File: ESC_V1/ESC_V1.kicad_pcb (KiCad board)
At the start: 2 copper layers, 58.2 x 22.2 mm, 19 parts, among them J1 Conn_01x07_Female, J2 Conn_01x01_Female, J3 Conn_01x01_Female, J4 Conn_01x01_Female, J5 Conn_01x01_Female, J6 Conn_01x01_Female, Q1 BSP129, Q11 P Channel 40V 30A, Q2 BSP129, Q3 P Channel 40V 30A, Q4 BSP129, Q7 P Channel 40V 30A, U1 ULN2803A

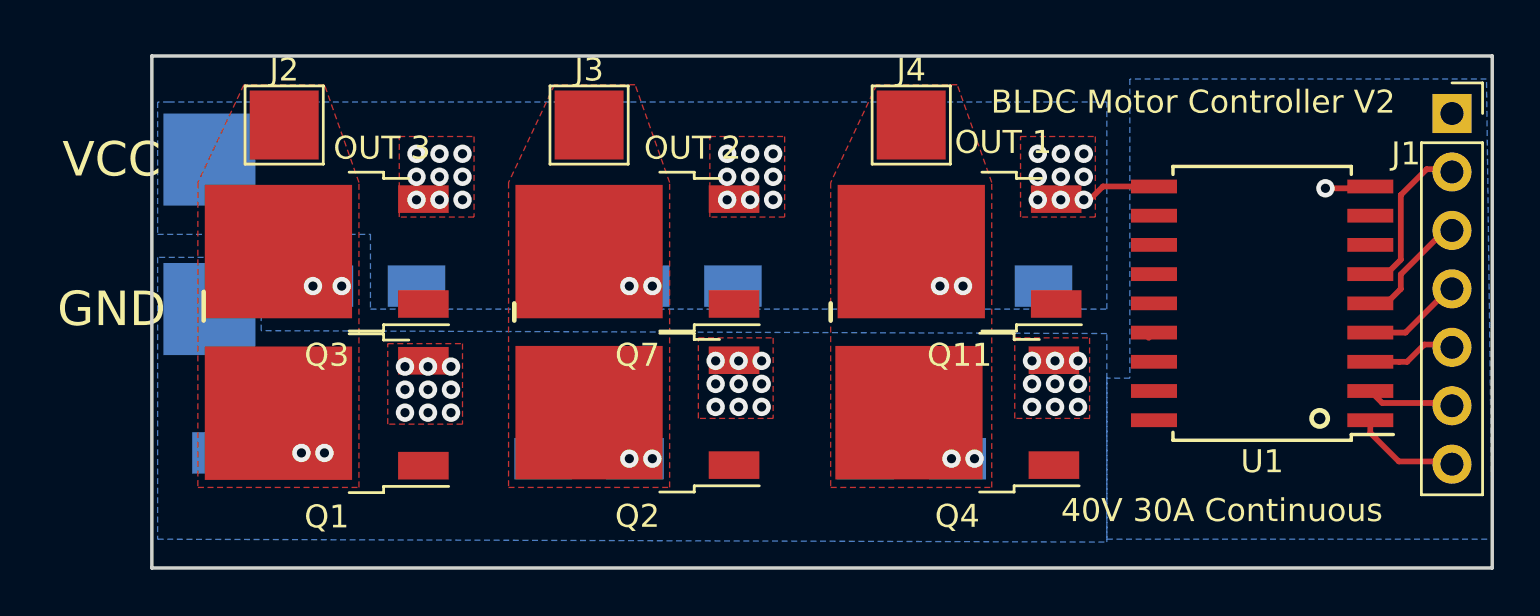
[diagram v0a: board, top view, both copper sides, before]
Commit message: Fixing git issues
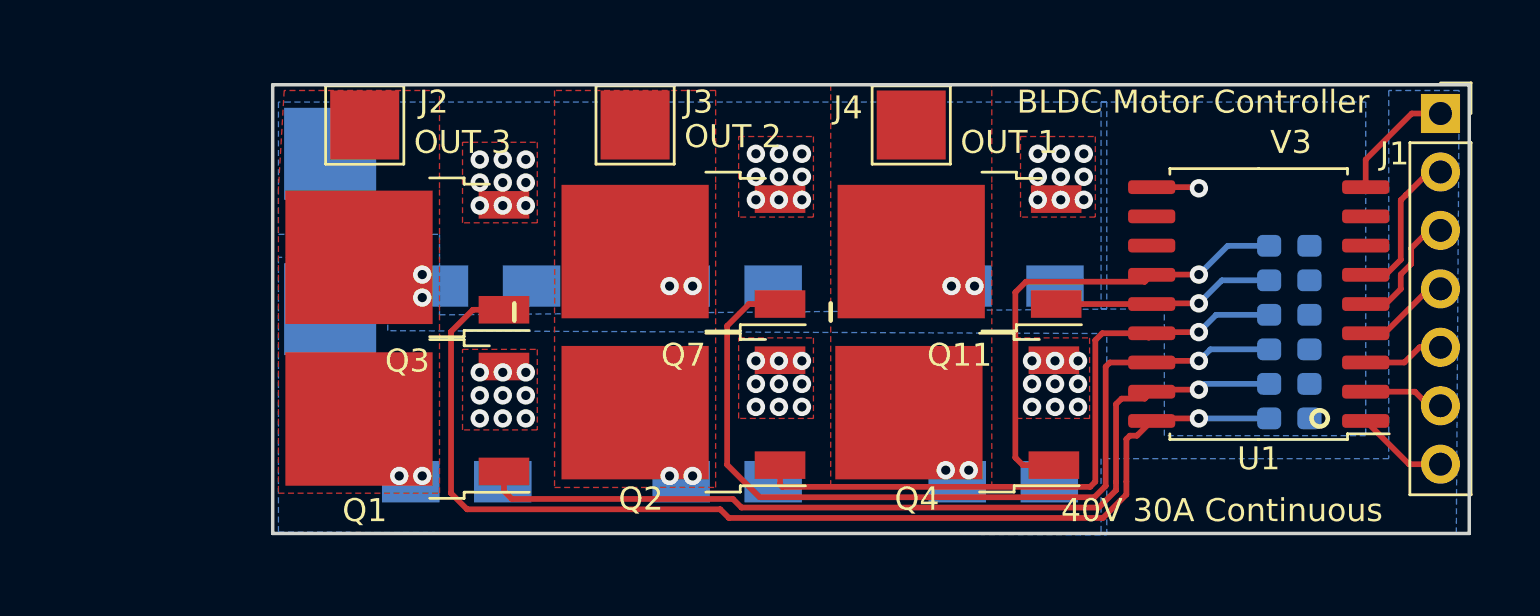
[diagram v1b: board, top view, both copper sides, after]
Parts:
- added R1: 100 ohm, Resistor_SMD:R_0603_1608Metric_Pad1.05x0.95mm_HandSolder, B.Cu at (176.2, 64.2)
- added R2: 100 ohm, Resistor_SMD:R_0603_1608Metric_Pad1.05x0.95mm_HandSolder, B.Cu at (176.2, 62.8)
- added R3: 100 ohm, Resistor_SMD:R_0603_1608Metric_Pad1.05x0.95mm_HandSolder, B.Cu at (176.2, 61.2)
- added R4: 100 ohm, Resistor_SMD:R_0603_1608Metric_Pad1.05x0.95mm_HandSolder, B.Cu at (176.2, 59.8)
- added R5: 100 ohm, Resistor_SMD:R_0603_1608Metric_Pad1.05x0.95mm_HandSolder, B.Cu at (176.2, 58.2)
- added R6: 100 ohm, Resistor_SMD:R_0603_1608Metric_Pad1.05x0.95mm_HandSolder, B.Cu at (176.2, 56.8)
- moved D2 8.34 mm to (140.0, 67.0), turned to 0 degrees
- moved D4 6.08 mm to (151.8, 67.0), turned to 0 degrees
- moved J5 5.26 mm to (134.5, 52.8)
- moved J6 5.25 mm to (134.5, 59.5)
- moved D1 5.00 mm to (141.2, 58.5)
- moved D6 4.12 mm to (163.8, 67.0), turned to 0 degrees
- moved Q1 3.51 mm to (137.8, 64.3)
- moved Q3 3.51 mm to (137.8, 57.2)
- moved J2 3.50 mm to (136.0, 51.5)
- moved J3 2.00 mm to (147.8, 51.5)
- moved Q2 2.00 mm to (149.8, 64.0)
- moved Q7 2.00 mm to (149.8, 57.0)
- moved D3 1.75 mm to (151.8, 58.5)
- moved D5 0.50 mm to (164.0, 58.5)
- moved J1 0.50 mm to (182.8, 51.0)
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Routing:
- net OUT1: track 0.00 -> 48.9 mm, vias 0 -> 1
- net OUT2: track 0.00 -> 38.8 mm, vias 0 -> 1
- net OUT3: track 0.00 -> 38.6 mm, vias 0 -> 1
- net OUT4: track 0.33 -> 29.2 mm, vias 0 -> 1
- net OUT6: track 0.00 -> 20.9 mm, vias 0 -> 1
- net OUT5: track 0.00 -> 9.68 mm, vias 0 -> 1
- net GND: track 1.98 -> 5.39 mm, vias 28 -> 27
- net VCC: track 4.29 -> 2.07 mm, vias 27 -> 28
- net Net-(J1-Pad2): track 7.08 -> 5.91 mm
- net Net-(J1-Pad7): track 4.61 -> 3.53 mm
- net Net-(J1-Pad4): track 4.39 -> 3.55 mm
- net Net-(J1-Pad5): track 3.86 -> 3.02 mm
- net Net-(J1-Pad6): track 3.77 -> 3.00 mm
- net Net-(J1-Pad3): track 5.28 -> 4.64 mm
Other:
- board size 58.2 x 22.2 mm -> 52 x 19.5 mm
- board text added: "1"
- board text added: "2"
- board text added: "3"
- board text added: "BLDC Motor Controller"
- board text added: "V3"
- board text removed: "BLDC Motor Controller V2"
